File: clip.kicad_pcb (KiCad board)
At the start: 2 copper layers, 42.9 x 52.1 mm, 38 parts, among them Q1 2.5A/30V, U1 MCP73831, U2 AP2112K-3.3, U3 ESP32-WROOM-32

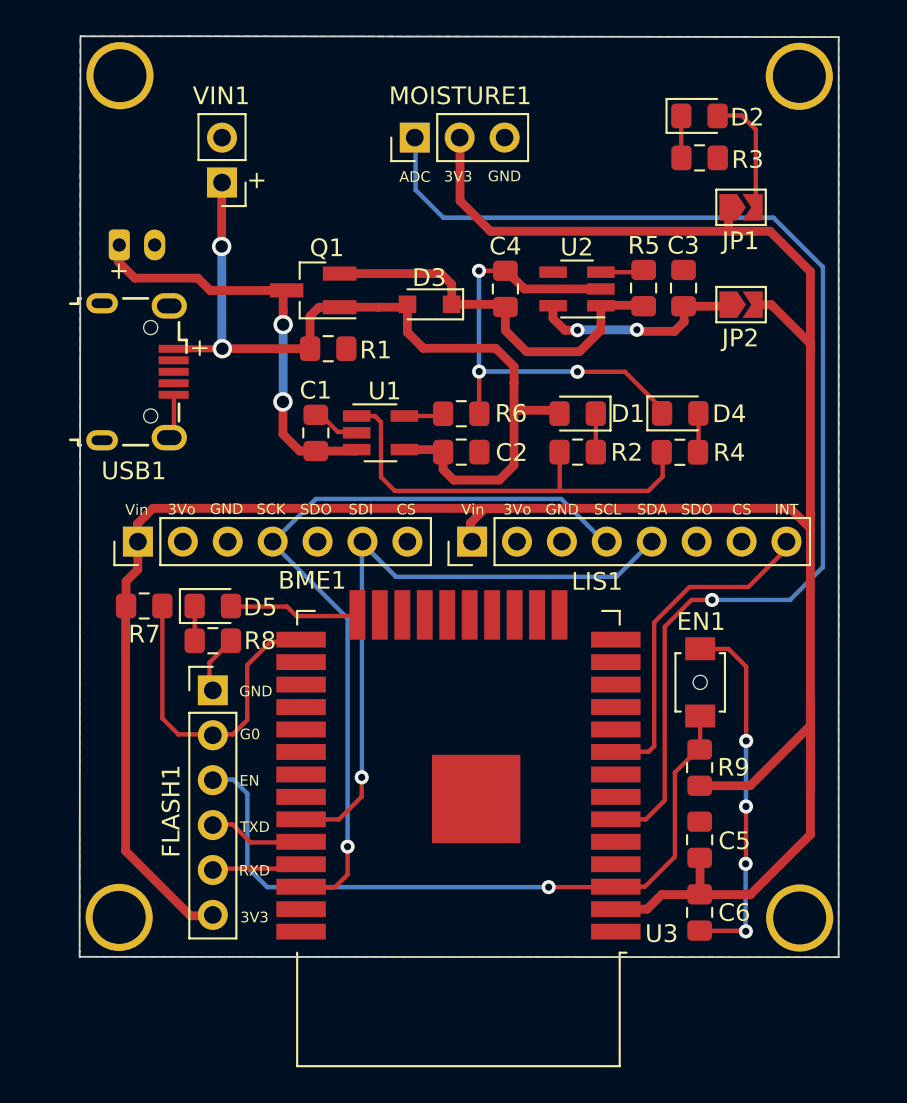
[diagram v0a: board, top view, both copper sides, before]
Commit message: Bump design
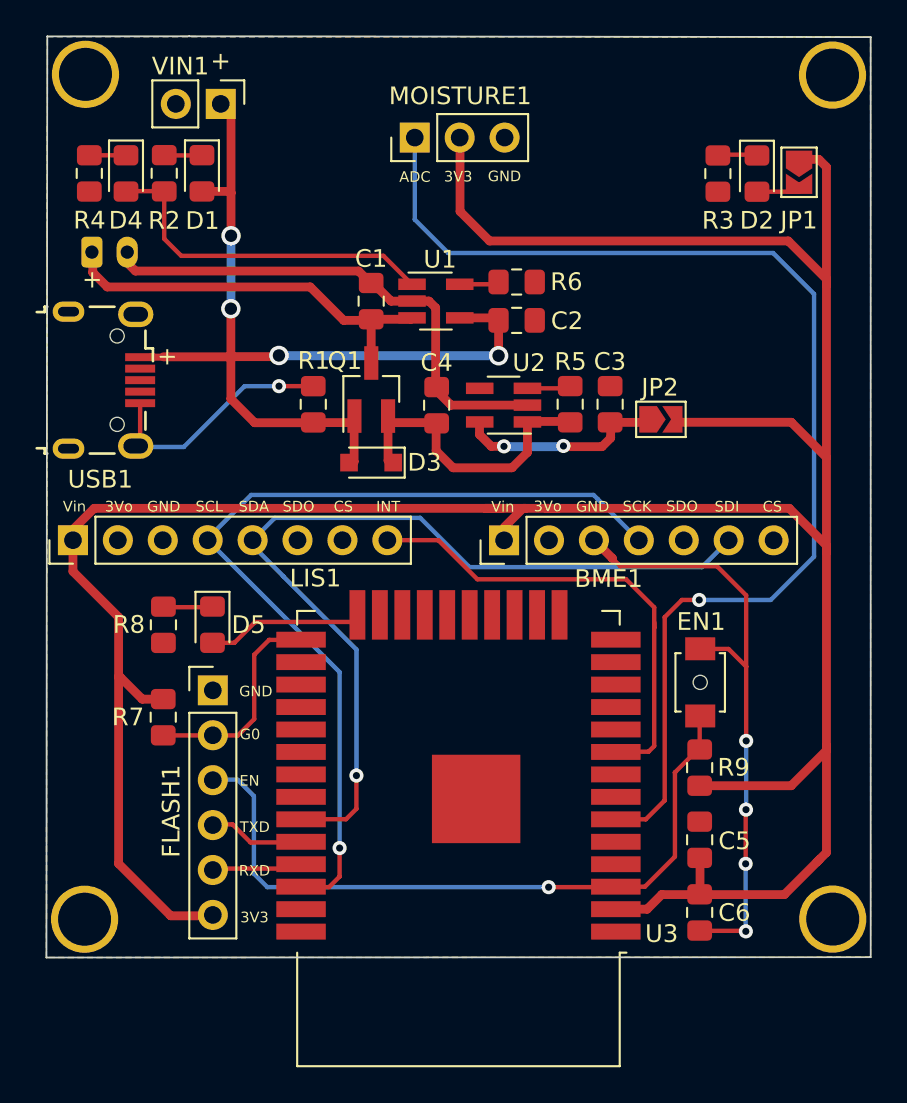
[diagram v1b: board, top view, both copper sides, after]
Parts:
- moved R4 36.9 mm to (128.0, 81.0), turned to 90 degrees
- moved D4 34.2 mm to (130.0, 81.0), turned to 270 degrees
- moved R2 28.2 mm to (132.2, 81.0), turned to 90 degrees
- moved D1 25.2 mm to (134.3, 81.0), turned to 270 degrees
- moved LIS1 22.6 mm to (127.0, 101.7)
- moved BME1 20.7 mm to (151.4, 101.7)
- moved D3 9.54 mm to (143.9, 97.3)
- moved C1 8.08 mm to (143.9, 88.2)
- moved U1 8.08 mm to (147.6, 88.2)
- moved C2 8.08 mm to (152.1, 89.3)
- moved R6 8.08 mm to (152.1, 87.1)
- moved JP2 7.92 mm to (160.3, 94.9)
- moved U2 7.77 mm to (151.4, 94.1)
- moved C3 7.77 mm to (157.4, 94.0)
- moved R5 7.77 mm to (155.1, 94.0)
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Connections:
- D4 pad 1: GND -> Net-(D4-Pad1)
- R2 pad 1: Net-(R2-Pad1) -> Net-(D4-Pad2)
- R4 pad 1: Net-(D4-Pad2) -> GND
- R4 pad 2: Net-(R2-Pad1) -> Net-(D4-Pad1)
- U1 pad 1: Net-(R2-Pad1) -> Net-(D4-Pad2)
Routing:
- net Net-(R2-Pad1): track 24.6 -> 0.00 mm
- net GND: track 56.8 -> 79.5 mm, vias 7 -> 5
- net +3V3: track 160.3 -> 178.8 mm
- net Net-(D4-Pad2): track 2.33 -> 20.0 mm
- net SDA: track 36.3 -> 50.6 mm
- net INT: track 18.6 -> 26.9 mm
- net VBUS: track 47.9 -> 55.8 mm, vias 2 -> 4
- net SCL: track 45.7 -> 52.1 mm
- net IO0: track 18.9 -> 12.6 mm
- net Net-(C4-Pad1): track 21.8 -> 16.2 mm
- net Net-(D2-Pad2): track 7.43 -> 2.39 mm
- net Net-(D4-Pad1): track 0.00 -> 2.08 mm
- net IO2: track 7.29 -> 8.68 mm
- net +BATT: track 24.8 -> 23.7 mm, vias 2 -> 0
- net ADC1: track 68.5 -> 67.6 mm
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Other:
- board size 42.9 x 52.1 mm -> 46.6 x 52.1 mm
